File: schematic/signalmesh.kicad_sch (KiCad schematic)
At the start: 131 parts, among them J1 FPGA I/O, J10 INA219_CONFIG, J11 INA219_CONFIG, J12 AAM_DBG, J13 DSM_DBG, J14 ACM_DBG, J15 INA219_CONFIG, J16 DSM_DBG, J17 LCD_display, J2 FPGA I/O, J3 LCD_display, J4 TDM_DBG, J5 INA219_CONFIG, J6 INA219_CONFIG, J7 INA219_CONFIG, J8 FPGA I/O, J9 FPGA I/O, U1 NUCLEO-H753ZI, U10 INA219AxD, U11 INA219AxD, U12 INA219AxD, U13 INA219AxD, U14 W25Q128JVS, U15 AP2112K-3.3, U16 74HC4050D, U17 NUCLEO-H753ZI, U18 HDSP-7503, U19 HDSP-7503, U2 HDSP-7503, U20 INA219AxD, U21 74HC4050D, U22 AP2112K-3.3, U23 W25Q128JVS, U24 74HC4050D, U25 AP2112K-3.3, U26 W25Q128JVS, U27 MCP2551-I-P, U28 74LVC1G3157, U29 MCP2551-I-P, U3 NUCLEO-F303RE, U30 MCP2551-I-P, U31 MCP2551-I-P, U4 YAAJ_BluePill_Part_Like, U5 24LC256-I_SN, U6 BME280, U7 INA219AxD, U8 24LC256-I_SN, U9 NUCLEO-F446RE

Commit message: CAN rework
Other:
- note added: "AAM CAN TLM"
- note added: "DSM CAN TLM"
- note added: "TDM CAN TLM"
- note added: "UUM CAN TLM"
- note removed: "AAM CAN DBG"
- note removed: "DSM CAN DBG"
- note removed: "TDM CAN DBG"
- note removed: "UUM CAN DBG"
- moved on the sheet: C10, C8, C9, D19, D25, D26, D27, J13, R1, R10, R42, R43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

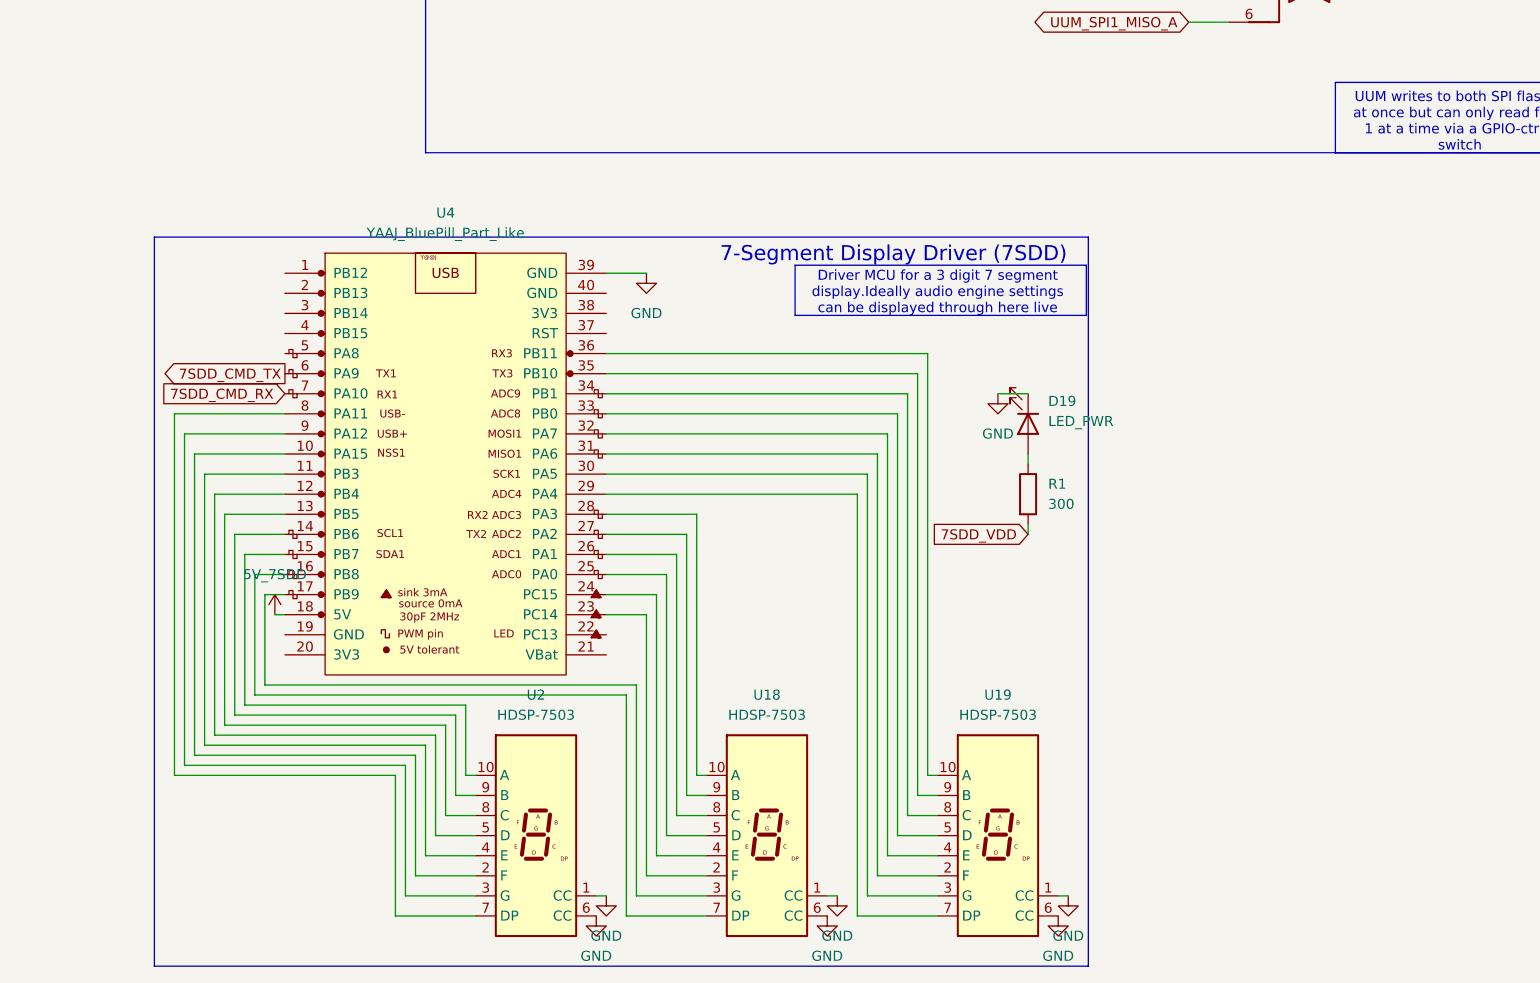
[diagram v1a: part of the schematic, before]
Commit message: PCB updates
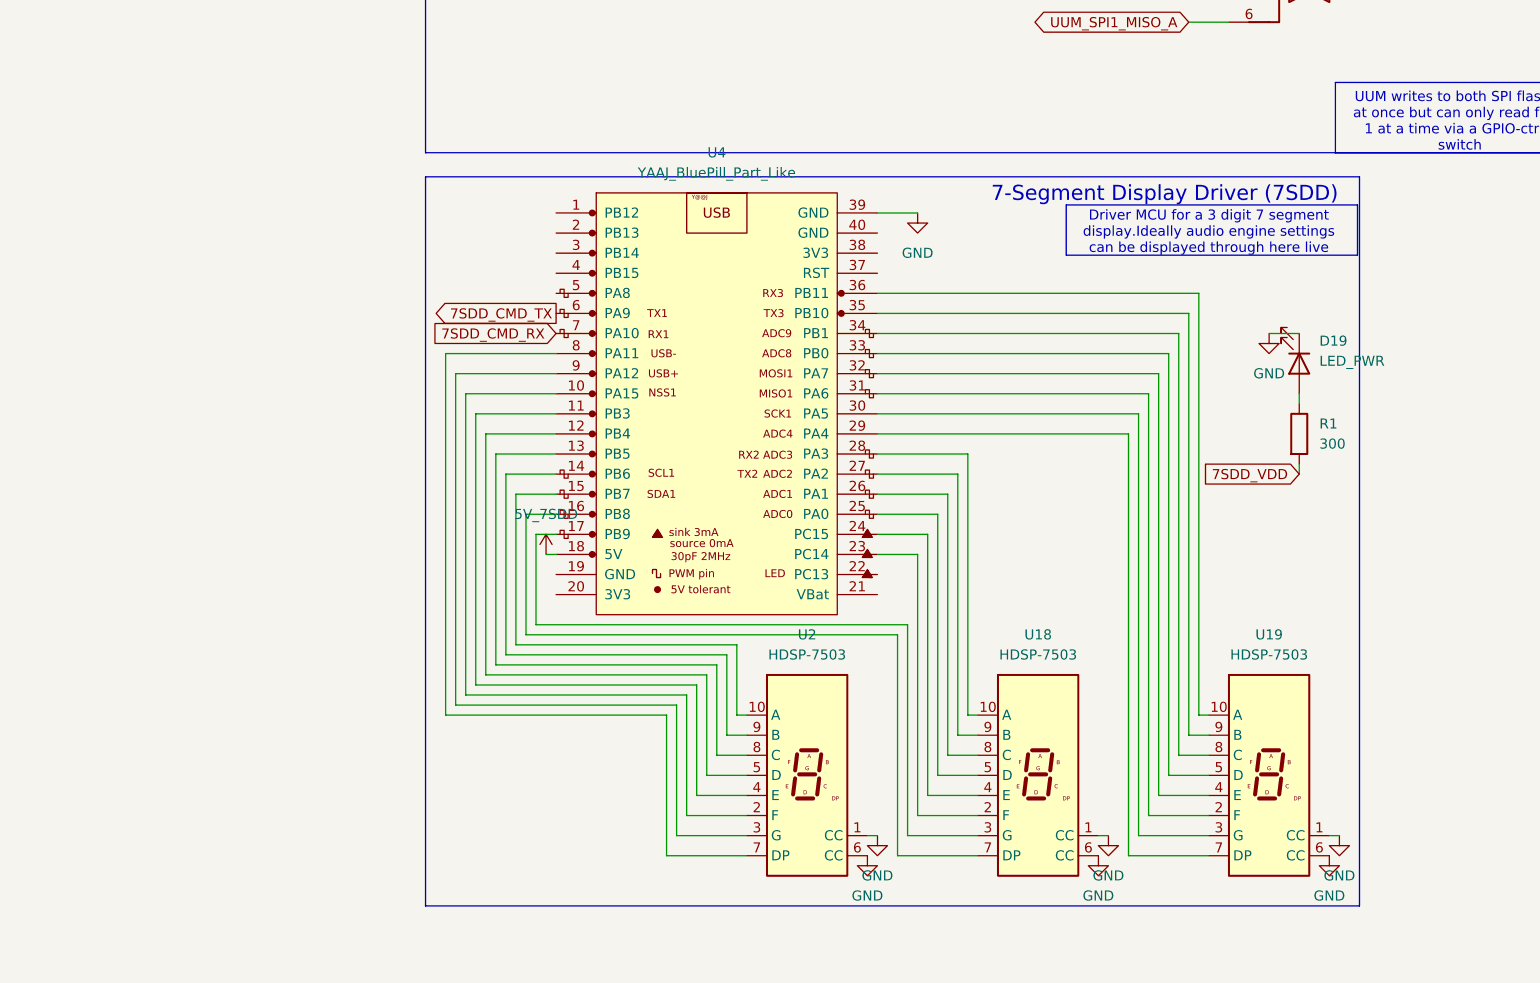
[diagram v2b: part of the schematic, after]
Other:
- moved on the sheet: D19, R1, U18, U19, U2, U4
